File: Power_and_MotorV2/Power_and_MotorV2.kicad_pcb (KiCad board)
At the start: 2 copper layers, 110 x 110 mm, 25 parts, among them J1 Barrel_Jack_Switch_Pin3Ring, M1 Motor_DC, Q1 BC337, Q2 BC337, SW1 SW_DPDT_x2, U1 LM317_TO-220, U2 Pin-Connector, U3 Pin-Connector, U4 Pin-Connector, U5 Pin-Connector, U6 Pin-Connector, U7 Pin-Connector

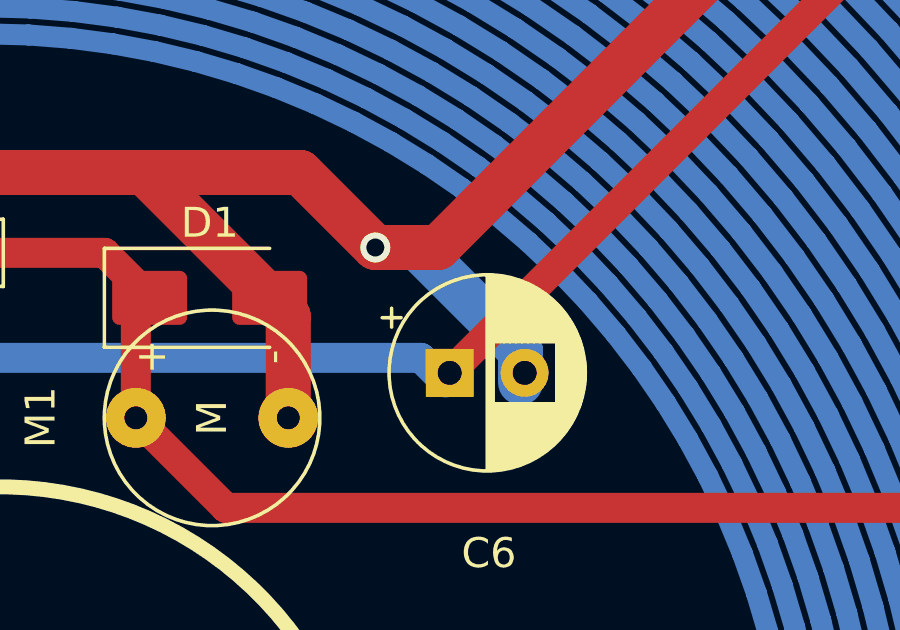
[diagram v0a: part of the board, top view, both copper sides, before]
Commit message: FinalV1
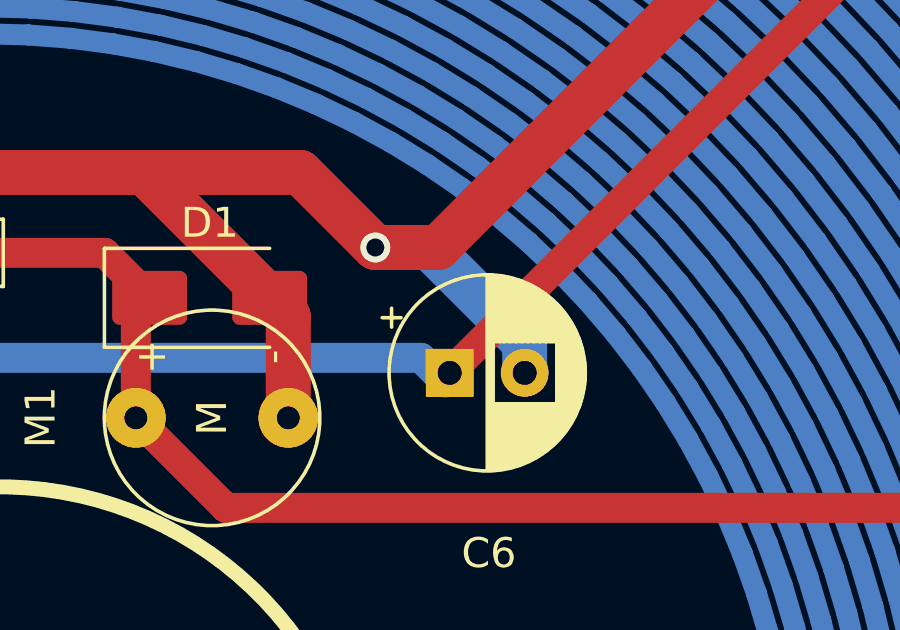
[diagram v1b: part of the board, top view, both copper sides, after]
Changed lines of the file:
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@@
-	)
-	(segment
-		(start 162.521434 79.821419)
-		(end 163.915343 79.821419)
-		(width 1.5)
-		(layer "B.Cu")
-		(net "GND")
 	)
 	(segment
 		(start 109.08 131.539985)
 		(end 109.08 135)
-		(width 1.5)
-		(layer "B.Cu")
-		(net "GND")
-	)
-	(segment
-		(start 167.361434 83.26751)
-		(end 167.361434 84.321419)
 		(width 1.5)
 		(layer "B.Cu")
@@
 		(start 111.361434 56.321419)
 		(end 111.361434 66.138566)
+		(width 1.5)
+		(layer "B.Cu")
+		(net "GND")
+	)
+	(segment
+		(start 164.321419 79.821419)
+		(end 167.5 83)
 		(width 1.5)
 		(layer "B.Cu")
@@
 	)
 	(segment
+		(start 162.521434 79.821419)
+		(end 164.321419 79.821419)
+		(width 1.5)
+		(layer "B.Cu")
+		(net "GND")
+	)
+	(segment
+		(start 167.5 83)
+		(end 167.5 84)
+		(width 1.5)
+		(layer "B.Cu")
+		(net "GND")
+	)
+	(segment
 		(start 109.08 136)
 		(end 116.08 143)
@@
 		(width 1.5)
 		(layer "B.Cu")
-		(net "GND")
-	)
-	(segment
-		(start 163.915343 79.821419)
-		(end 167.361434 83.26751)
-		(width 1.5)
-		(layer "B.Cu")
